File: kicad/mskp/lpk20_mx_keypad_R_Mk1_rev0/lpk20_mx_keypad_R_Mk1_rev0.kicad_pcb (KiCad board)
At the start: 2 copper layers, 122 x 97 mm, 25 parts, among them J1 Conn_01x12_Socket, SW1 Switch, SW10 Switch, SW2 Switch, SW3 Switch, SW4 Switch, SW5 Switch, SW6 Switch, SW7 Switch, SW8 Switch, SW9 Switch

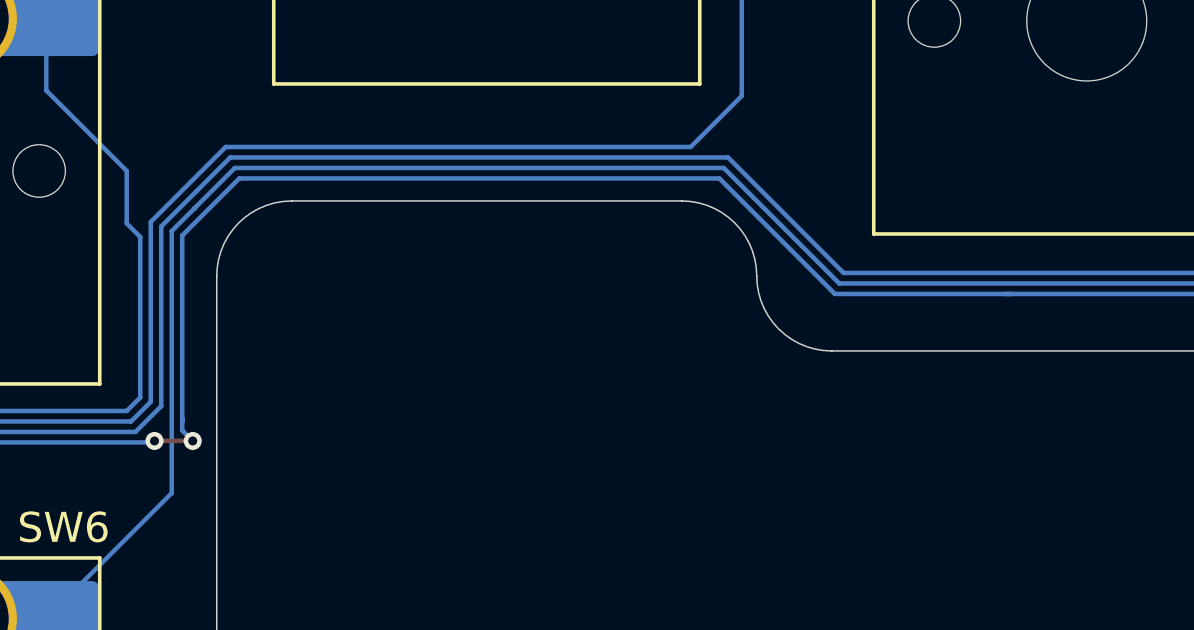
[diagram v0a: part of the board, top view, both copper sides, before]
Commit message: Final tweaks to PCBs before second round of mskp fabrications
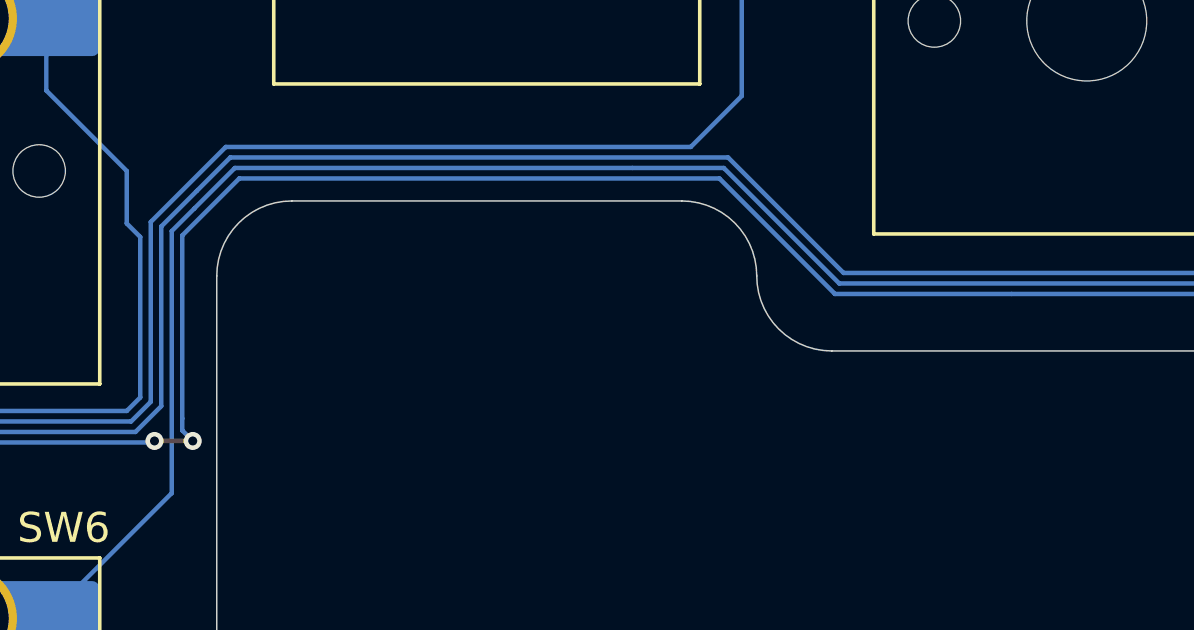
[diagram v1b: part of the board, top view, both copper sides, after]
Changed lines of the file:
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@@
 			(plot_on_all_layers_selection 0x0000000_00000000)
 			(disableapertmacros no)
-			(usegerberextensions no)
-			(usegerberattributes yes)
-			(usegerberadvancedattributes yes)
-			(creategerberjobfile yes)
+			(usegerberextensions yes)
+			(usegerberattributes no)
+			(usegerberadvancedattributes no)
+			(creategerberjobfile no)
 			(dashed_line_dash_ratio 12.000000)
 			(dashed_line_gap_ratio 3.000000)
 			(svgprecision 4)
 			(plotframeref no)
-			(viasonmask no)
+			(viasonmask yes)
 			(mode 1)
 			(useauxorigin no)
@@
 			(psa4output no)
 			(plotreference yes)
-			(plotvalue yes)
+			(plotvalue no)
 			(plotfptext yes)
 			(plotinvisibletext no)
 			(sketchpadsonfab no)
-			(subtractmaskfromsilk no)
+			(subtractmaskfromsilk yes)
 			(outputformat 1)
 			(mirror no)
-			(drillshape 1)
+			(drillshape 0)
 			(scaleselection 1)
-			(outputdirectory "")
+			(outputdirectory "lpk20_r_mk1_exports")
 		)
 	)
@@
 	)
 	(segment
-		(start 143.85 77.25)
-		(end 143.85 77.35)
-		(width 0.15)
-		(layer "B.Cu")
-		(net 15)
-	)
-	(segment
 		(start 123.694974 78.05)
 		(end 142.875 78.05)
@@
 	)
 	(segment
-		(start 171.5 73.1)
-		(end 171.279253 73.1)
-		(width 0.15)
-		(layer "B.Cu")
-		(net 15)
-	)
-	(segment
 		(start 119.32 103.92)
 		(end 122.5 100.74)
@@
 		(width 0.15)
 		(layer "B.Cu")
-		(net 20)
-	)
-	(segment
-		(start 144.252513 70.252513)
-		(end 144.25 70.255026)
-		(width 0.15)
-		(layer "B.Cu")

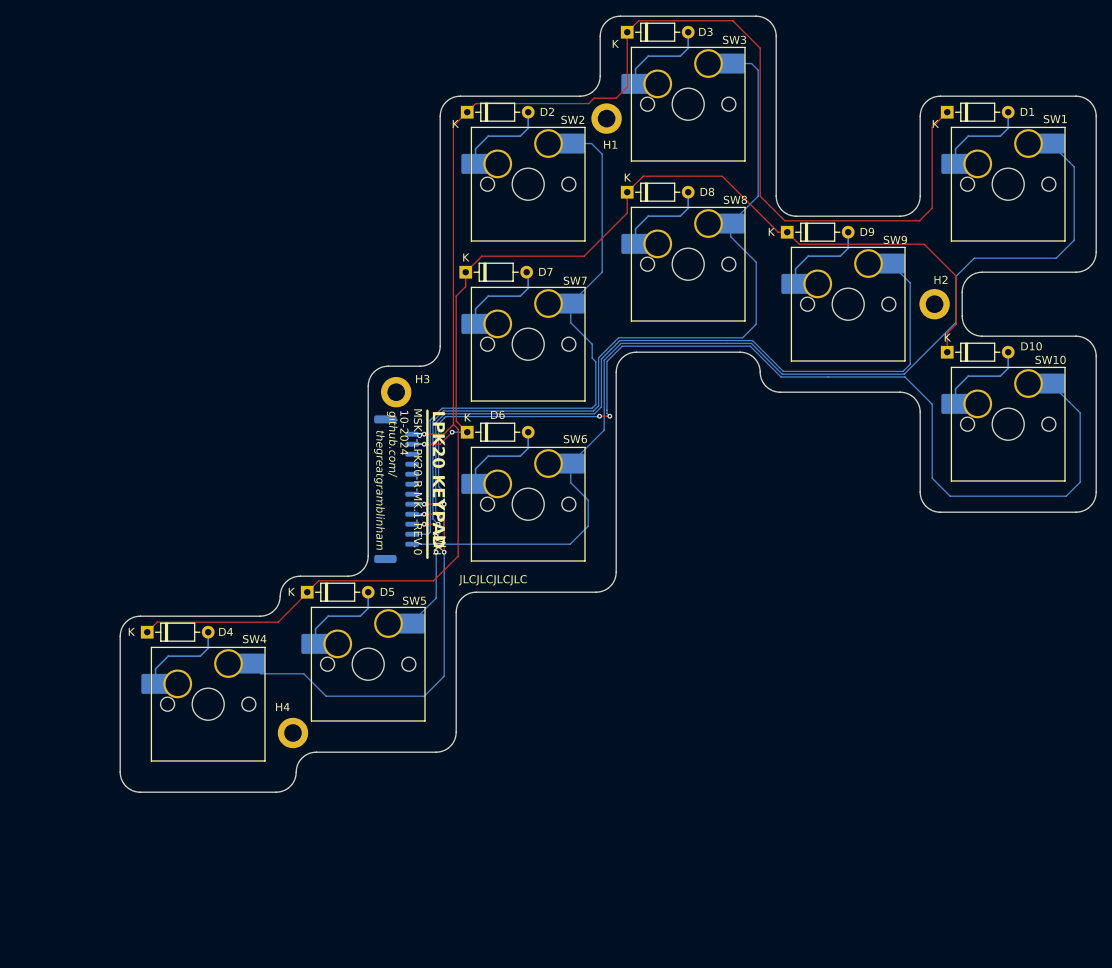
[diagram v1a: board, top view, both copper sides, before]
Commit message: Updates mskp pcbs with case design layers
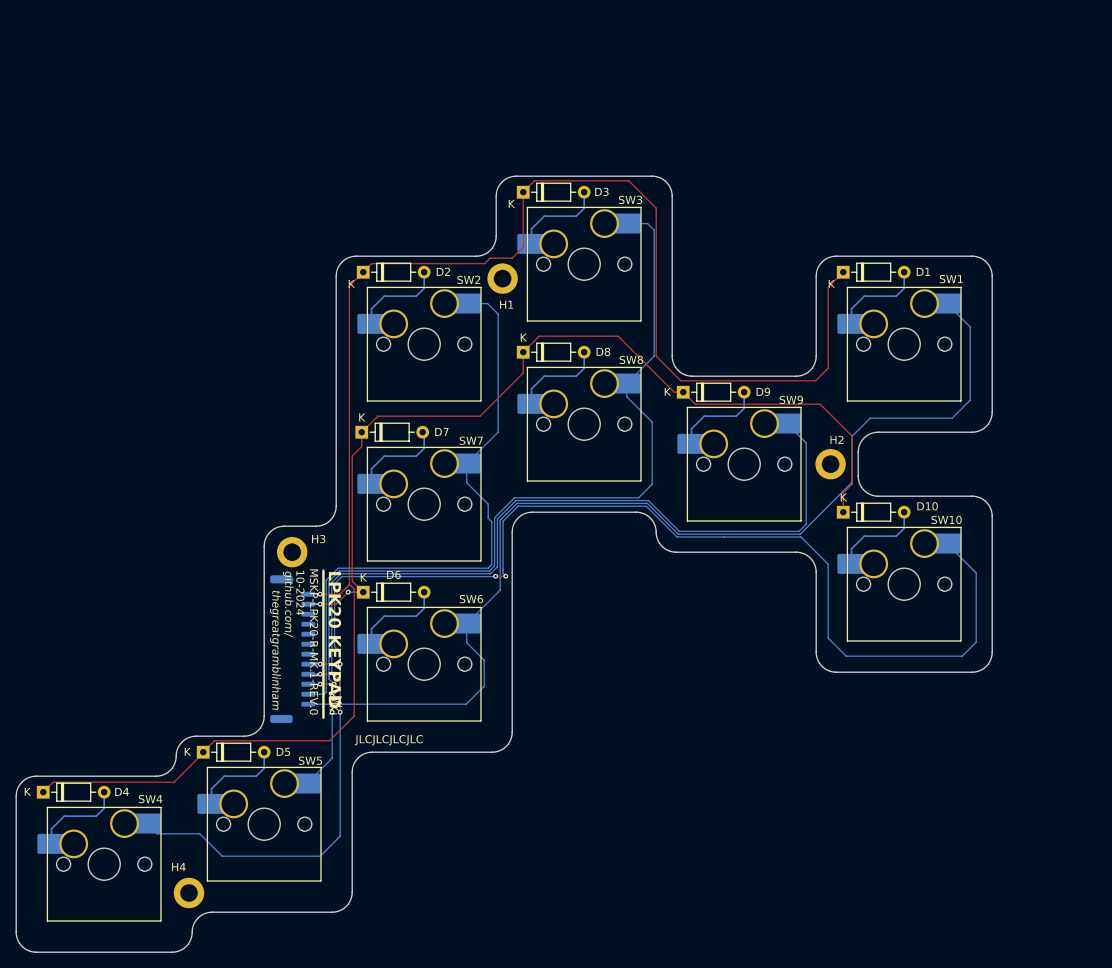
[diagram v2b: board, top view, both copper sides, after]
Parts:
- moved D1 23.9 mm to (173.4, 60.0)
- moved D10 23.9 mm to (173.4, 90.0)
- moved D2 23.9 mm to (113.4, 60.0)
- moved D3 23.9 mm to (133.4, 50.0)
- moved D4 23.9 mm to (73.4, 125.0)
- moved D5 23.9 mm to (93.4, 120.0)
- moved D6 23.9 mm to (113.4, 100.0)
- moved D7 23.9 mm to (113.2, 80.0)
- moved D8 23.9 mm to (133.4, 70.0)
- moved D9 23.9 mm to (153.4, 75.0)
- moved H1 23.9 mm to (130.8, 60.8)
- moved H2 23.9 mm to (171.8, 84.0)
- moved H3 23.9 mm to (104.5, 95.0)
- moved H4 23.9 mm to (91.6, 137.6)
- moved J1 23.9 mm to (104.5, 107.1)
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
